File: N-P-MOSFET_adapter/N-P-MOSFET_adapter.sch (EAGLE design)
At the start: 13 parts, among them Q1 BSS83P, Q2 BSS83P, Q3 BSS138, Q4 BSS138

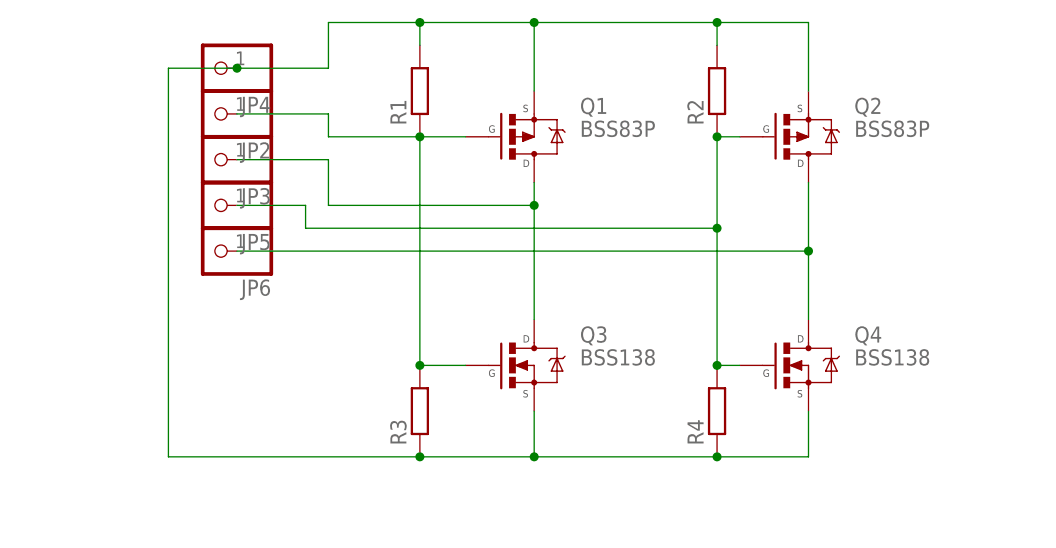
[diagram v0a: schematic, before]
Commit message: schematic
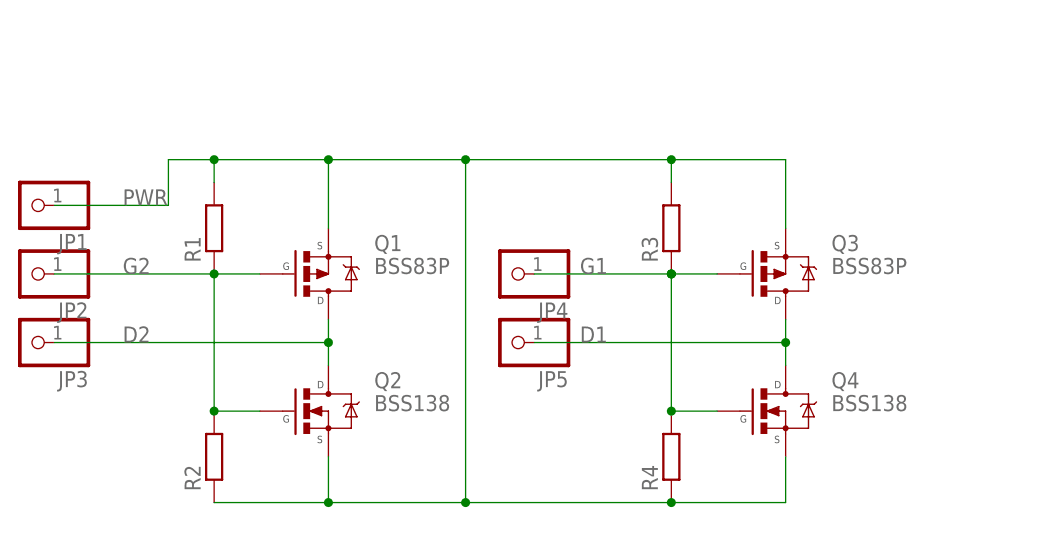
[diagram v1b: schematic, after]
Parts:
- removed JP6: (no value), my-pinhead:PINHD-1X1JUST_PIN
- added JP1: (no value), my-pinhead:PINHD-1X1JUST_PIN
- Q2: value BSS83P -> BSS138; device my-mosfet:BSS83P -> my-mosfet:BSS138
- Q3: value BSS138 -> BSS83P; device my-mosfet:BSS138 -> my-mosfet:BSS83P
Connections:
- net D1: now also JP5.1, Q3.D; no longer JP6.1, Q2.D
- net D2: now also Q2.D; no longer Q3.D
- net G1: now also JP4.1, Q3.G, R3.1; no longer JP5.1, Q2.G, R2.1
- net G2: now also Q2.G, R2.2; no longer Q3.G, R3.2
- net PWR: now also JP1.1, R2.1, R3.2; no longer JP4.1, R2.2, R3.1
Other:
- moved on the sheet: JP2, JP3, JP4, JP5, Q1, Q2, Q3, Q4, R1, R2, R3, R4

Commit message: new adapters
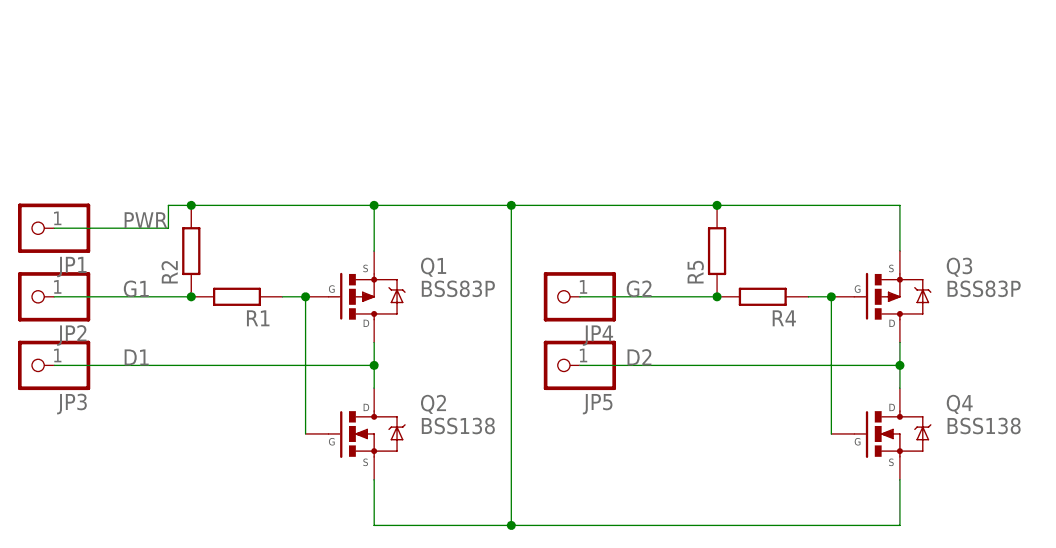
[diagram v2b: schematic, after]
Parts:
- removed R3: (no value), rcl:R-EU_R0805
- added R5: (no value), rcl:R-EU_R0805
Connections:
- new net N$3: Q1.G, Q2.G, R1.1
- new net N$4: Q3.G, Q4.G, R4.1
- net D1: now also JP3.1, Q1.D, Q2.D; no longer JP5.1, Q3.D, Q4.D
- net D2: now also JP5.1, Q3.D, Q4.D; no longer JP3.1, Q1.D, Q2.D
- net G1: now also JP2.1, R1.2, R2.1; no longer JP4.1, Q3.G, Q4.G, R3.1, R4.2
- net G2: now also JP4.1, R4.2, R5.1; no longer JP2.1, Q1.G, Q2.G, R1.1, R2.2
- net PWR: now also R2.2, R5.2; no longer R1.2, R2.1, R3.2, R4.1
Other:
- moved on the sheet: JP1, JP2, JP3, JP4, JP5, Q1, Q2, Q3, Q4, R1, R2, R4
